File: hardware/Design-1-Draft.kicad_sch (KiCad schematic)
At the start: 32 parts, among them J1 Barrel_Jack_Switch, M1 WATERPUMP-1, M2 WATERPUMP-2, Q1 IRLZ44N, Q2 IRLZ44N, SW1 Button, U3 ADS1115IDGS, U5 Tang_Nano_9K

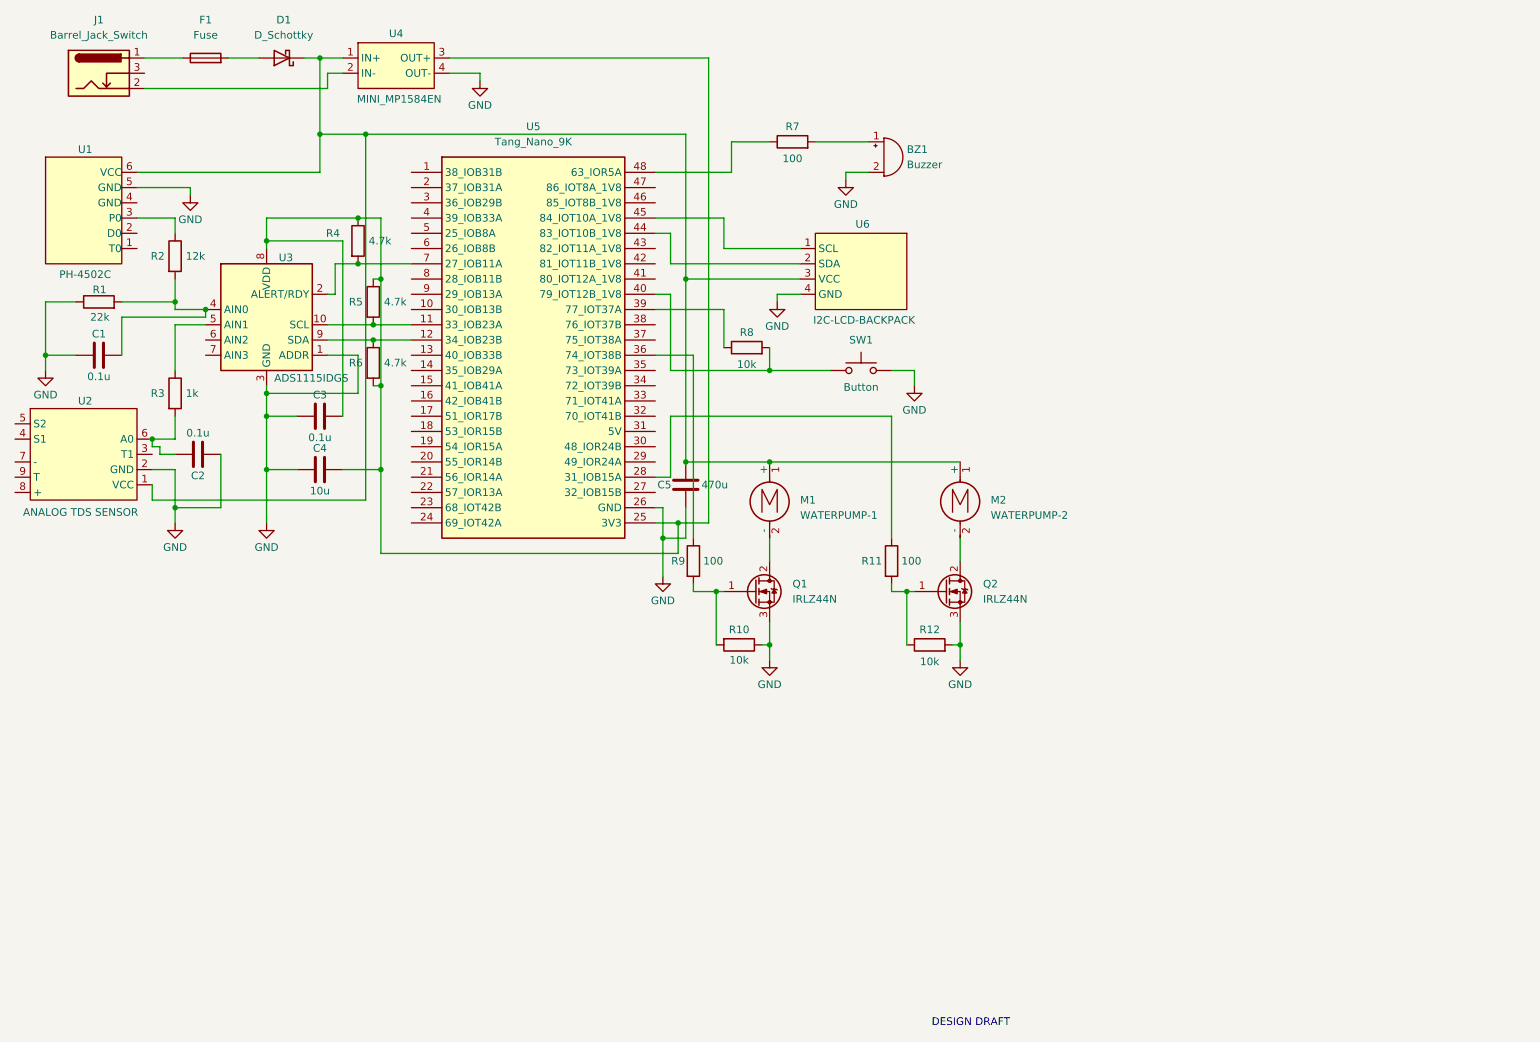
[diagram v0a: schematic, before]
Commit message: modified schem, wala pang pcb
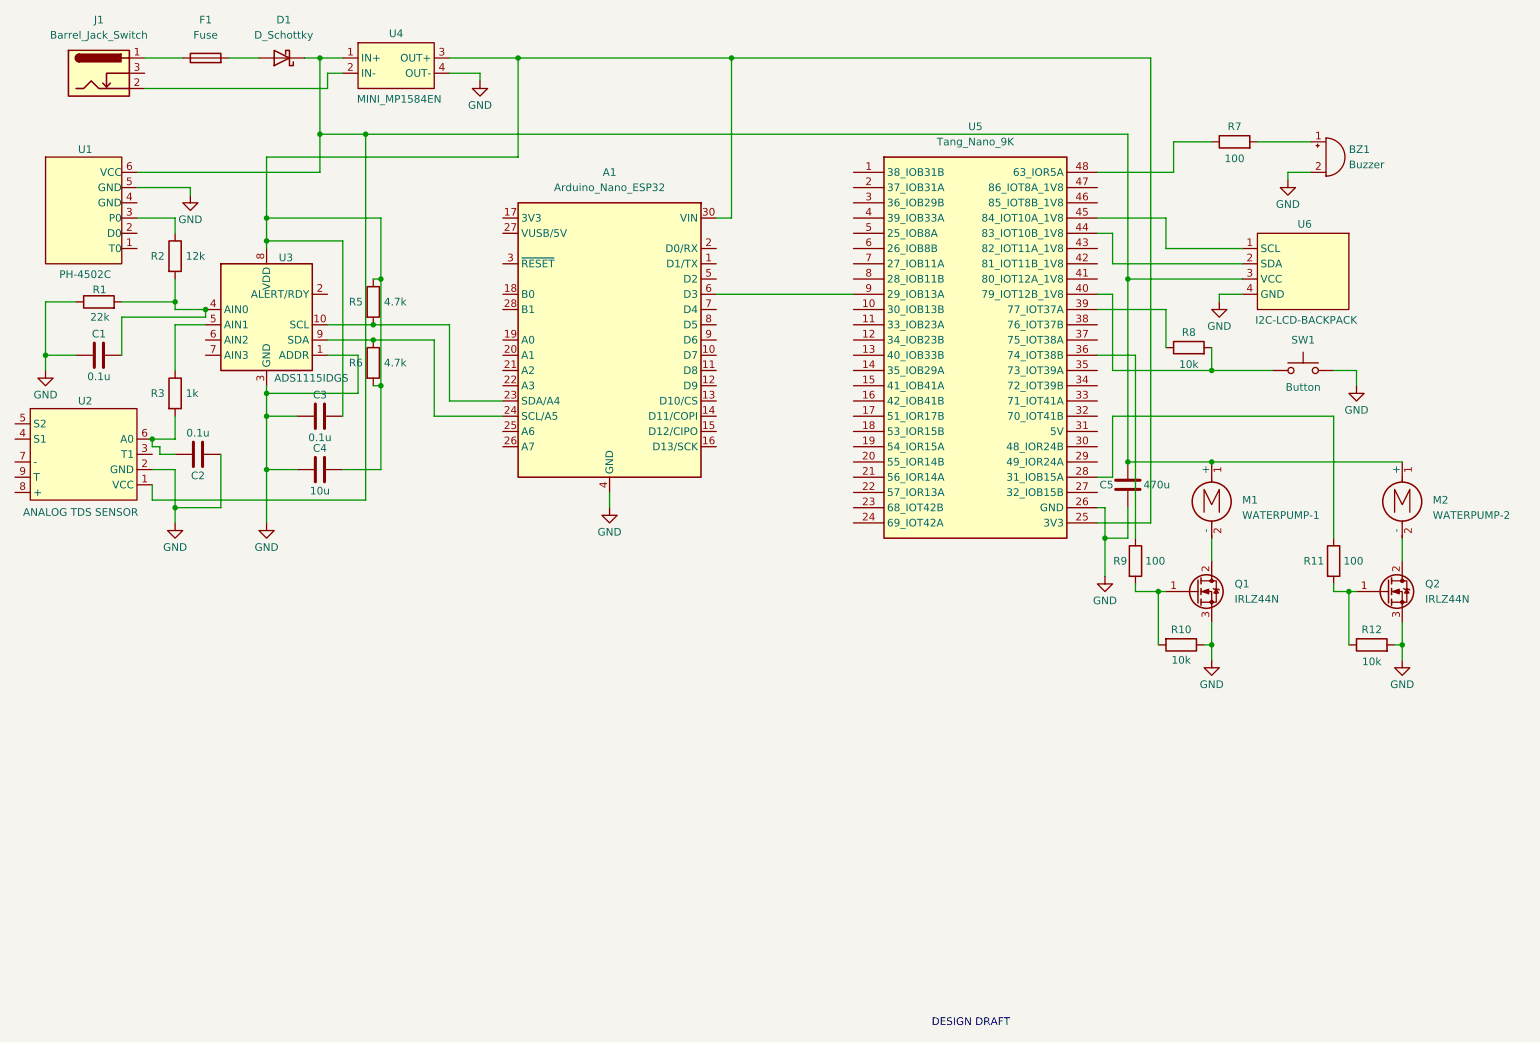
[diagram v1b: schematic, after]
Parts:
- removed R4: 4.7k, Resistor_THT:R_Axial_DIN0207_L6.3mm_D2.5mm_P10.16mm_Horizontal, symbol Device:R
- added A1: Arduino_Nano_ESP32, Module:Arduino_Nano, symbol MCU_Module:Arduino_Nano_ESP32
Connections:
- net GND: now also A1.29 (GND), A1.4 (GND)
- net at C3.2, C4.2, R5.1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: now also A1.30 (VIN)
- net at R5.2, U3.10 (SCL): now also A1.23 (SDA/A4); no longer U5.11 (33_IOB23A)
- net at U5.7 (27_IOB11A): no longer U3.2 (ALERT/RDY)
- net at R6.1, U3.9 (SDA): now also A1.24 (SCL/A5); no longer U5.12 (34_IOB23B)
- net at U5.9 (29_IOB13A): now also A1.6 (D3)
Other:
- moved on the sheet: BZ1, C5, M1, M2, Q1, Q2, R10, R11, R12, R7, R8, R9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
